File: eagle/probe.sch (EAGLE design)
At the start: 14 parts

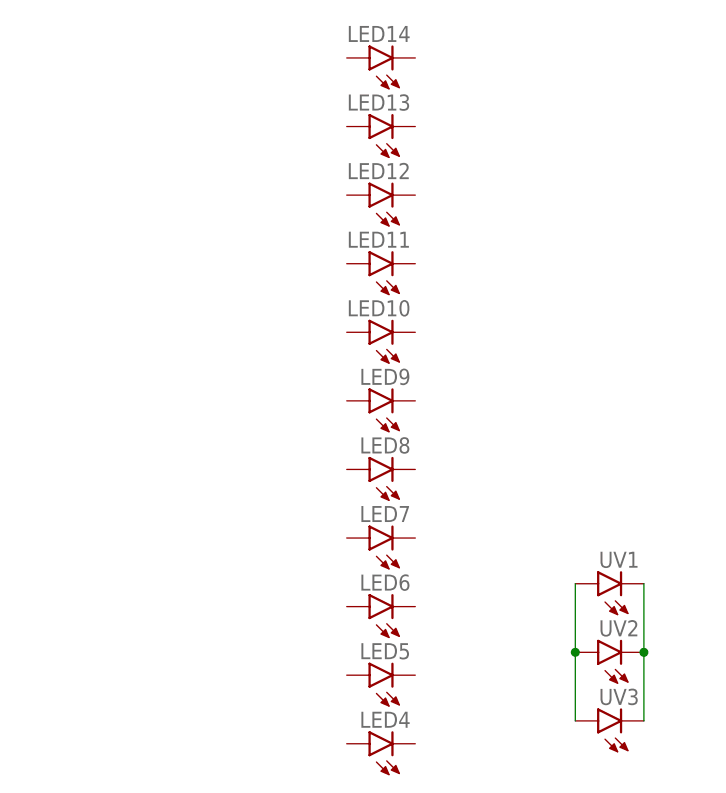
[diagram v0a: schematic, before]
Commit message: probe pcb v1
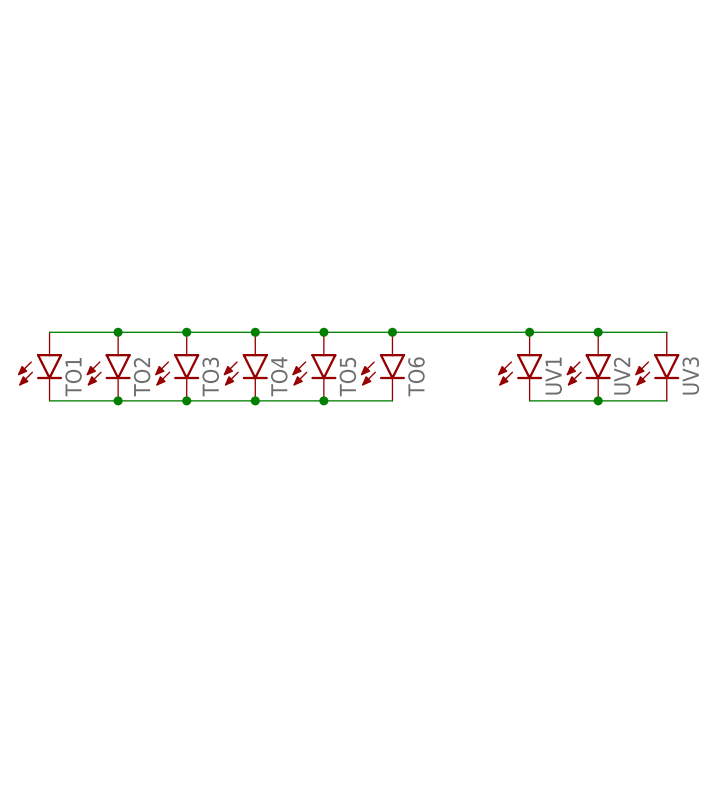
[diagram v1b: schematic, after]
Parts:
- removed LED10, LED11, LED12, LED13, LED14, LED4, LED5, LED6, LED7, LED8, LED9: (no value), led:LED5MM
- added TO1, TO2, TO3, TO4, TO5, TO6: (no value), general:LED5MM
- UV1, UV2, UV3: device led:LED5MM -> general:LED5MM
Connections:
- new net N$2: TO1.C, TO2.C, TO3.C, TO4.C, TO5.C, TO6.C
- net N$1: now also TO1.A, TO2.A, TO3.A, TO4.A, TO5.A, TO6.A
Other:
- moved on the sheet: UV1, UV2, UV3
